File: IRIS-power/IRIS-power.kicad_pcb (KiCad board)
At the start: 2 copper layers, 65 x 65 mm, 77 parts, among them J11 Powerpole, J13 Conn_01x20_MountingPin, J81 USB_C_Receptacle_USB2.0, Q21 2N7002, Q61 SSM3J328R, Q81 SSM3J328R, U21 MAX17261, U31 TPS2115APW, U41 LT3461A, U51 TPSM53604, U61 LTC3110, U62 PCA9537, U71 TLV75733PDBV, U81 TPD2E2U06, U82 STUSB4500LQTR

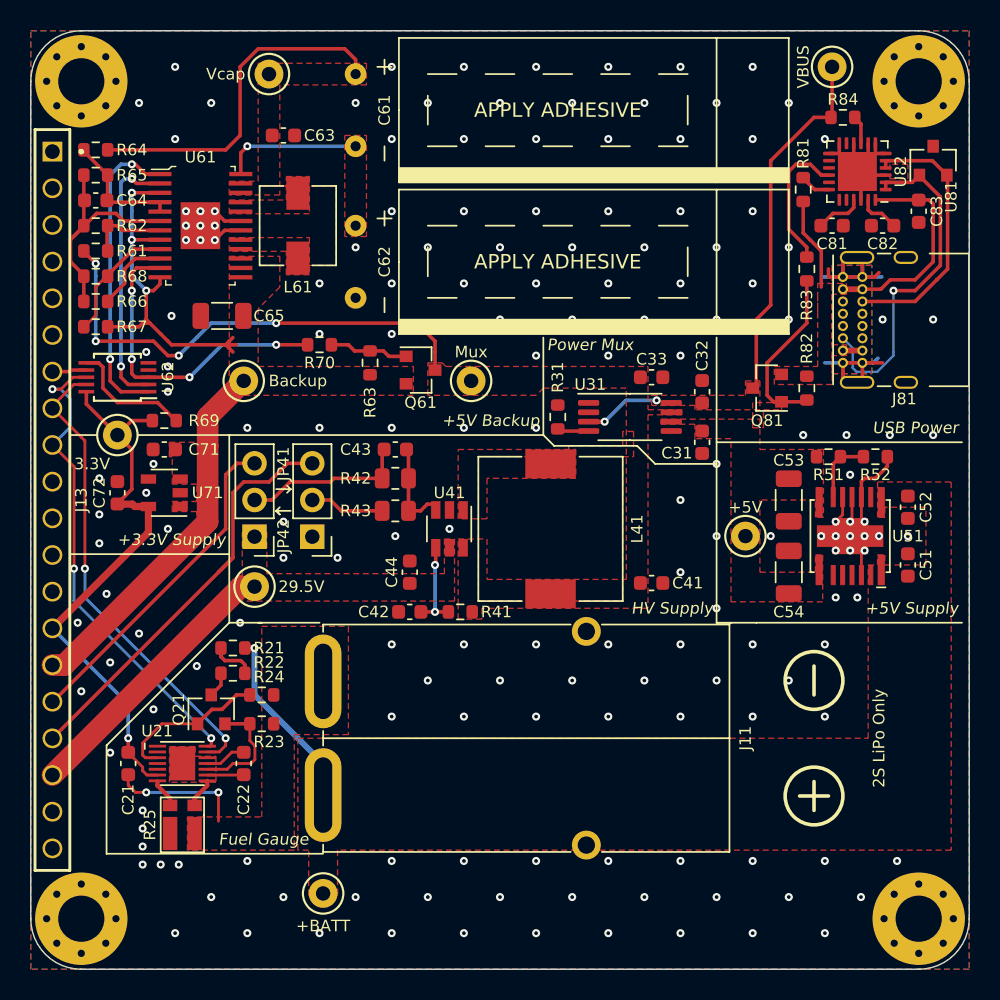
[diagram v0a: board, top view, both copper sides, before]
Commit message: Updated to V4.01
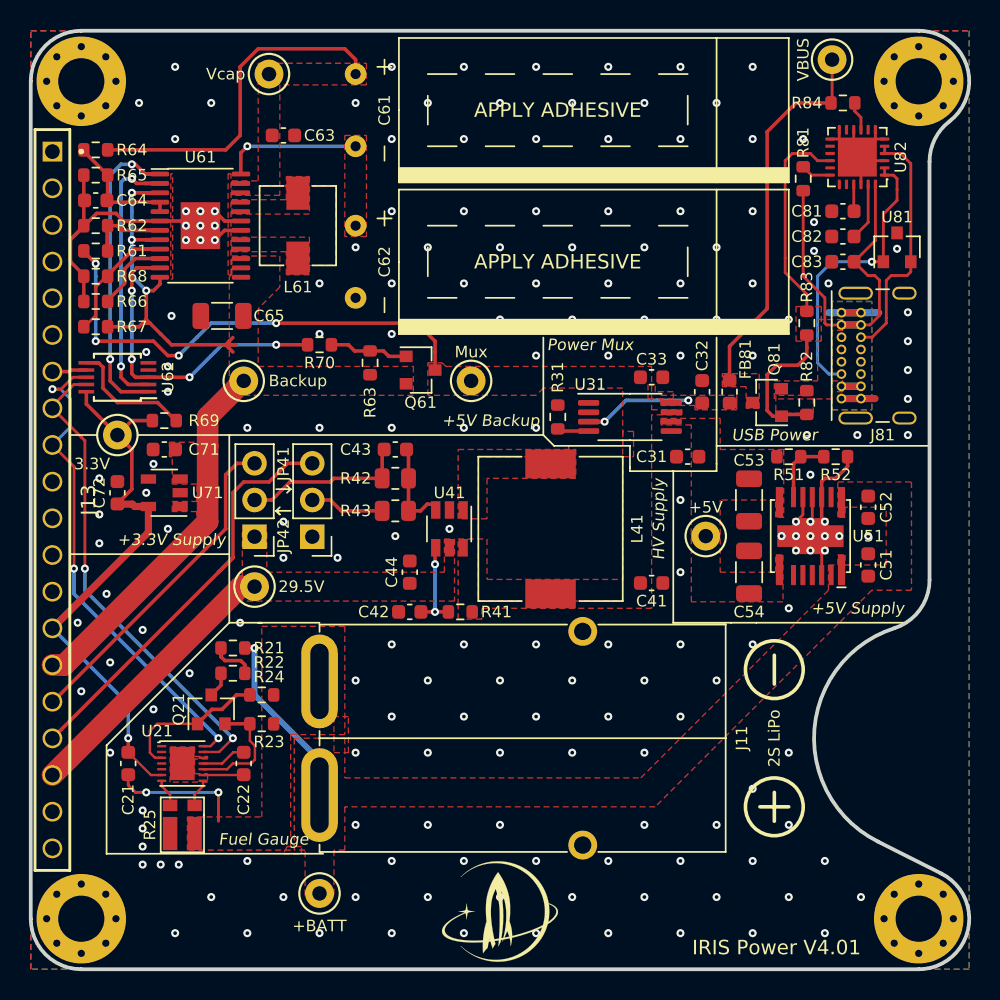
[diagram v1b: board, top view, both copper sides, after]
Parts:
- added FB81: Ferrite_Bead, Inductor_SMD:L_0603_1608Metric, F.Cu at (48.4, -7.50)
- added G***: LOGO, star-common-lib:star_8x7, F.Cu at (32.5, 28.5)
- J13: footprint star-common-lib:IRIS_Muons_physical -> star-common-lib:IRIS_V4_power
- J81: footprint Connector_USB:USB_C_Receptacle_GCT_USB4085 -> star-common-lib:USB_C_Receptacle_GCT_USB4085_Fixed
- R31: value 400R -> 402R
- U51: value TPSM53604 -> TPSM53602
- U82: footprint Package_DFN_QFN:QFN-24-1EP_4x4mm_P0.5mm_EP2.7x2.7mm -> star-common-lib:STUSB4500L
- moved U81 6.50 mm to (60.0, -17.5)
- moved C83 6.31 mm to (56.2, -16.5), turned to 180 degrees
- moved J81 6.02 mm to (62.2, -10.0)
- moved R83 3.75 mm to (53.8, -12.2)
- moved C82 2.85 mm to (56.2, -18.2)
- moved C51 2.75 mm to (58.0, 4.50)
- moved C52 2.75 mm to (58.0, 0.50)
- moved C53 2.75 mm to (49.8, 0.00)
- moved C54 2.75 mm to (49.8, 5.00)
- moved NT51 2.75 mm to (54.8, -0.94)
- moved R51 2.75 mm to (52.5, -3.00)
- moved R52 2.75 mm to (55.8, -3.00)
- moved TP102 2.75 mm to (46.8, 2.50)
- moved U51 2.75 mm to (54.0, 2.50)
- moved C31 1.41 mm to (45.5, -3.00), turned to 180 degrees
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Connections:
- J81 pad S1: GND -> Net-(J81-PadS1)
- Q81 pad 3: /Power Mux/VUSB -> Net-(FB81-Pad2)
- R84 pad 1: /Power Mux/VUSB -> Net-(FB81-Pad2)
- TP101 pad 1: /Power Mux/VUSB -> Net-(FB81-Pad2)
- U51 pad 6: Net-(U51-Pad6) -> GND
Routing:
- net Net-(FB81-Pad2): track 0.00 -> 26.6 mm
- net /Power Mux/VUSB: track 31.5 -> 8.53 mm
- net GND: track 52.5 -> 33.4 mm, vias 179 -> 187
- net /USB Connector/VBUS: track 23.2 -> 28.7 mm
- net Net-(R83-Pad2): track 9.82 -> 14.6 mm
- net /USB Connector/CC1: track 24.1 -> 20.5 mm
- net /3V Supply/VSYS: track 52.2 -> 54.3 mm
- net Net-(Q81-Pad1): track 12.1 -> 10.2 mm
- net Net-(C81-Pad1): track 3.34 -> 1.87 mm
- net /USB Connector/CC2: track 18.6 -> 17.2 mm
- net Net-(C82-Pad1): track 2.93 -> 4.01 mm
- net /5V Backup/FB: track 8.81 -> 9.87 mm
- net /5V Backup/~CMP_OUT: track 18.5 -> 19.6 mm
- net /5V Backup/DIR: track 5.55 -> 6.56 mm
- net /5V Backup/CAP_OK: track 21.3 -> 22.1 mm
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- added copper zone on F.Cu, net Net-(FB81-Pad2)
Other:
- outline, holes or cut-outs redrawn
- net class Low Clearance: clearance 0.2 -> 0.16
- rule pad_to_mask_clearance: 0.051 -> 0.0508
- board text added: "2S LiPo"
- board text added: "IRIS Power V4.01"
- board text removed: "2S LiPo Only"
